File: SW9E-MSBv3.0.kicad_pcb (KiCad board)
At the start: 2 copper layers, 105.5 x 93 mm, 18 parts, among them J1 22-05-3021, J2 22-05-3021, J3 90120-0763, J4 90120-0763, J6 SSW-104-03-F-S, J7 SSW-104-03-F-S, Q1 FDN5632N-F085, Q2 FDN5632N-F085, U1 MSP430FR2355TPTR

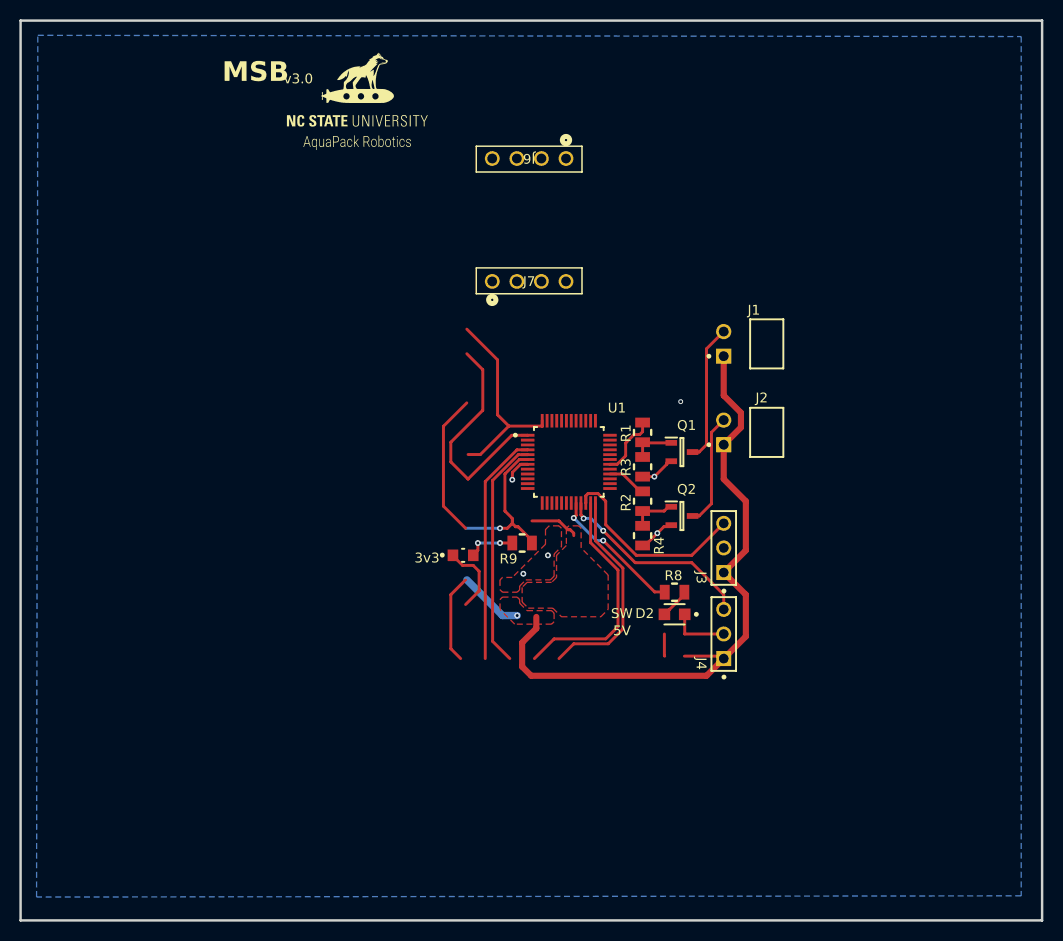
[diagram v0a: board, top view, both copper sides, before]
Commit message: Stuff
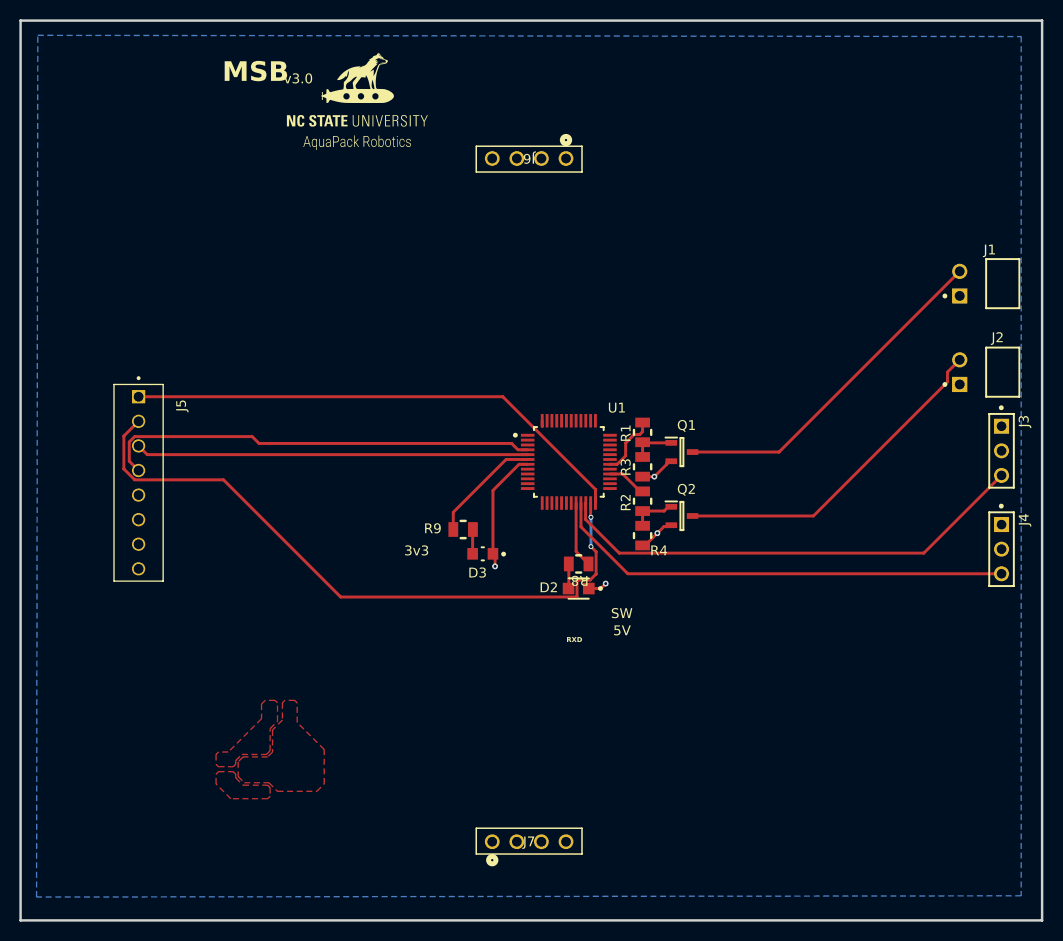
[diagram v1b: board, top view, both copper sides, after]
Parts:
- added J5: 640453-8, Library:TE_640453-8, F.Cu at (86.7, 88.1)
- moved J7 57.9 mm to (127.0, 134.1)
- moved J3 30.4 mm to (175.8, 93.7), turned to -90 degrees
- moved J4 30.0 mm to (175.8, 103.9), turned to -90 degrees
- moved J1 25.2 mm to (175.8, 76.4)
- moved J2 25.2 mm to (175.8, 85.6)
- moved R8 10.3 mm to (132.1, 105.4), turned to -90 degrees
- moved D2 10.3 mm to (132.1, 107.9)
- moved R9 6.25 mm to (120.2, 101.8), turned to -90 degrees
- moved D3 2.04 mm to (122.2, 104.3), turned to 180 degrees
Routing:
- net +5V: track 77.6 -> 0.00 mm
- net /TXD: track 23.9 -> 69.4 mm, vias 0 -> 2
- net /RXD: track 22.1 -> 52.6 mm
- net (no net): track 29.0 -> 0.00 mm, vias 1 -> 0
- net /SERVO1_CTRL: track 20.5 -> 49.4 mm
- net /SERVO2_CTRL: track 21.0 -> 47.9 mm, vias 2 -> 0
- net /SDA: track 23.8 -> 0.00 mm
- net Net-(Q2-D): track 11.6 -> 34.9 mm
- net /TST: track 24.0 -> 45.3 mm
- net Net-(Q1-D): track 14.2 -> 35.3 mm
- net /SCL: track 21.2 -> 0.55 mm
- net /RST: track 23.9 -> 40.6 mm
- net Net-(U1-P6.2/TB3.3): track 14.1 -> 6.82 mm, vias 2 -> 0
- net +3.3V: track 16.7 -> 11.7 mm, vias 1 -> 0
- net Net-(D3-A): track 5.02 -> 2.53 mm, vias 2 -> 0
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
